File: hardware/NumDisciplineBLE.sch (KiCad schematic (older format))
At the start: 22 parts, among them J2 SWD, J3 Ex_Bat, J4 Ex_USB, Q1 AO3407, Q2 AO3407, U1 E73-2G4M08S1C, U2 XC6220B331MR-G, U3 TP4054, U5 ATmega32A-P, X1 32.768kHz

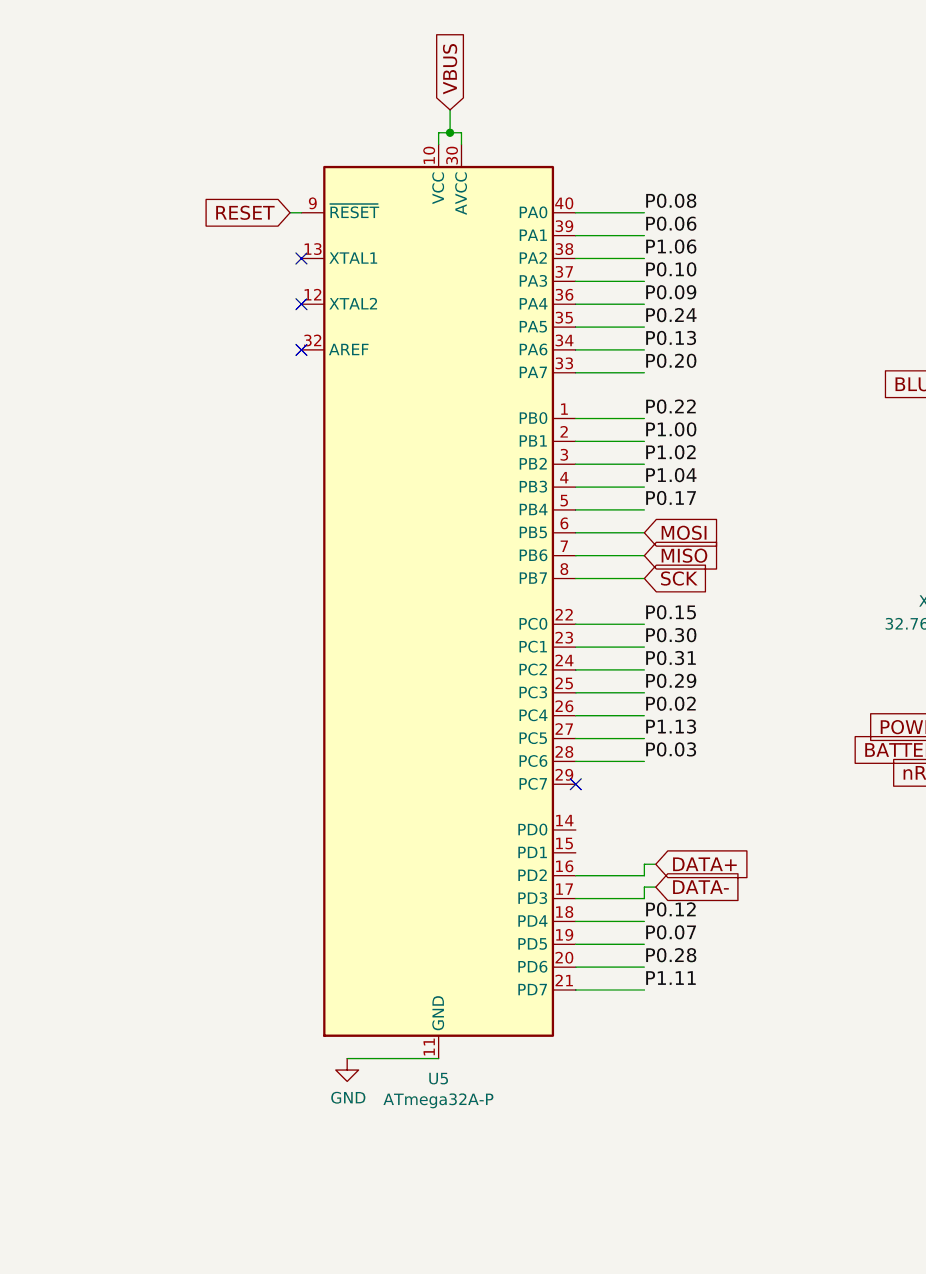
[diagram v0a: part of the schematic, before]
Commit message: basic layout done
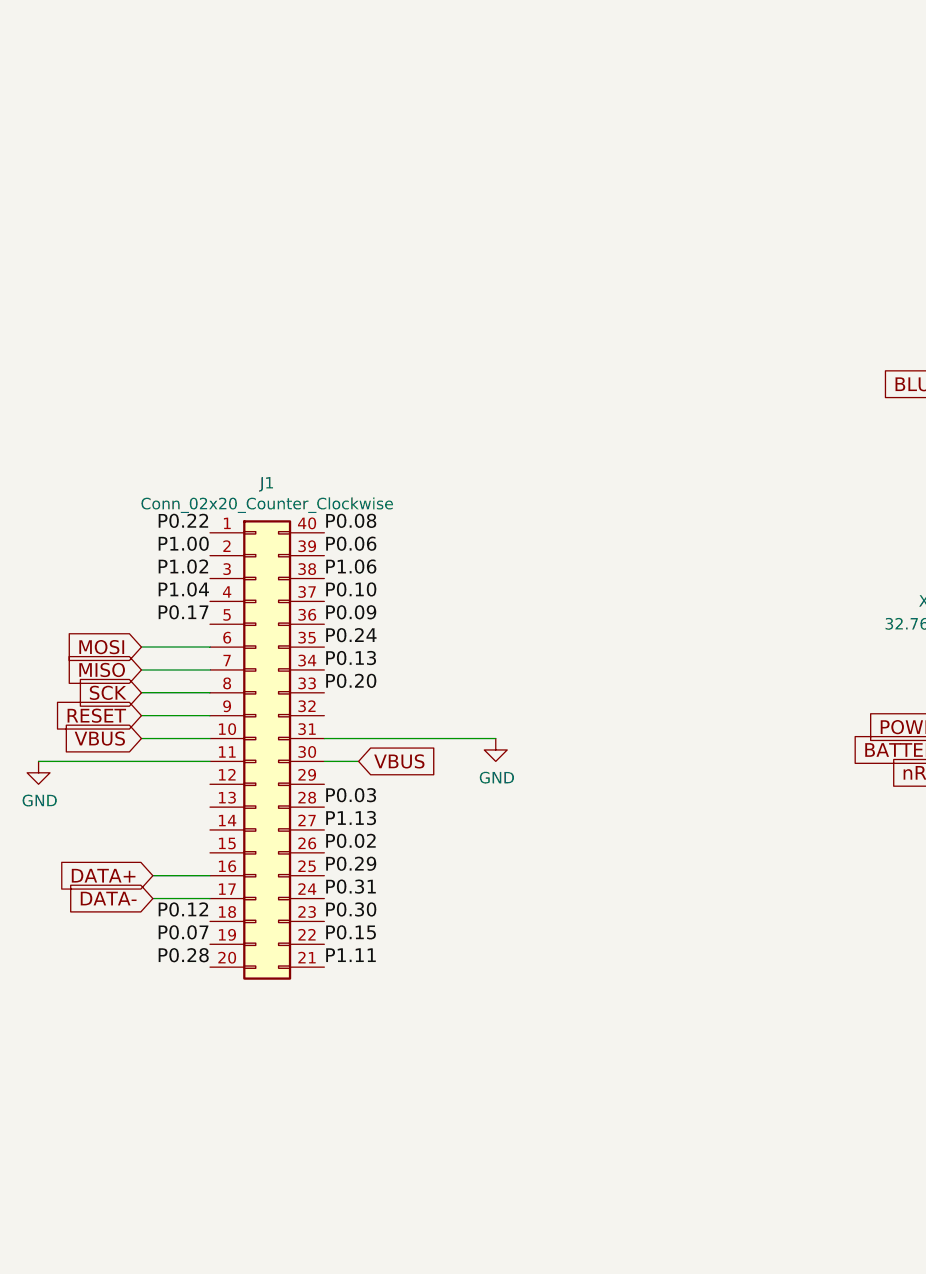
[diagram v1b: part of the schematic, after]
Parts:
- removed U5: ATmega32A-P, Package_DIP:DIP-40_W15.24mm, symbol MCU_Microchip_ATmega:ATmega32A-P
- added J1: Conn_02x20_Counter_Clockwise, nrfmicro:2x20_P2.54mm_Vertical_SMD_reversed, symbol Connector_Generic:Conn_02x20_Counter_Clockwise
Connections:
- net DATA+: now also J1.16 (Pin_16)
- net DATA-: now also J1.17 (Pin_17)
- net GND: now also J1.11 (Pin_11), J1.31 (Pin_31)
- net MISO: now also J1.7 (Pin_7)
- net MOSI: now also J1.6 (Pin_6)
- net P0.02: now also J1.26 (Pin_26)
- net P0.03: now also J1.28 (Pin_28)
- net P0.06: now also J1.39 (Pin_39)
- net P0.07: now also J1.19 (Pin_19)
- net P0.08: now also J1.40 (Pin_40)
- net P0.09: now also J1.36 (Pin_36)
- net P0.10: now also J1.37 (Pin_37)
- net P0.12: now also J1.18 (Pin_18)
- net P0.13: now also J1.34 (Pin_34)
- net P0.15: now also J1.22 (Pin_22)
- net P0.17: now also J1.5 (Pin_5)
- net P0.20: now also J1.33 (Pin_33)
- net P0.22: now also J1.1 (Pin_1)
- net P0.24: now also J1.35 (Pin_35)
- net P0.28: now also J1.20 (Pin_20)
- net P0.29: now also J1.25 (Pin_25)
- net P0.30: now also J1.23 (Pin_23)
- net P0.31: now also J1.24 (Pin_24)
- net P1.00: now also J1.2 (Pin_2)
- net P1.02: now also J1.3 (Pin_3)
- net P1.04: now also J1.4 (Pin_4)
- net P1.06: now also J1.38 (Pin_38)
- net P1.11: now also J1.21 (Pin_21)
- net P1.13: now also J1.27 (Pin_27)
- net RESET: now also J1.9 (Pin_9)
- net SCK: now also J1.8 (Pin_8)
- net VBUS: now also J1.10 (Pin_10), J1.30 (Pin_30)
- no-connect marks 4 -> 0
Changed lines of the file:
@@
 Wire Wire Line
 	3000 3050 3525 3050
+Wire Wire Line
+	-2150 2600 -2450 2600
+Wire Wire Line
+	-2450 2500 -2150 2500
+Wire Wire Line
+	-2150 2400 -2450 2400
+Wire Wire Line
+	-2450 2300 -2150 2300
+Text Label -2150 3500 2    60   ~ 0
+P0.12
+Text Label -2150 3600 2    60   ~ 0
+P0.07
+Text Label -2150 3700 2    60   ~ 0
+P0.28
+Text GLabel -2400 3400 0    60   Input ~ 0
+DATA-
+Text GLabel -2400 3300 0    60   Input ~ 0
+DATA+
 $Comp
-L MCU_Microchip_ATmega:ATmega32A-P U5
-U 1 1 5FA7B77E
-P -1150 2100
-F 0 "U5" H -1150 11  50  0000 C CNN
-F 1 "ATmega32A-P" H -1150 -80 50  0000 C CNN
-F 2 "Package_DIP:DIP-40_W15.24mm" H -1150 2100 50  0001 C CIN
-F 3 "http://ww1.microchip.com/downloads/en/DeviceDoc/atmel-8155-8-bit-microcontroller-avr-atmega32a_datasheet.pdf" H -1150 2100 50  0001 C CNN
-	1    -1150 2100
+L power:GND #PWR0111
+U 1 1 5FA32D25
+P -2900 2800
+F 0 "#PWR0111" H -2900 2550 50  0001 C CNN
+F 1 "GND" H -2895 2627 50  0000 C CNN
+F 2 "" H -2900 2800 50  0001 C CNN
+F 3 "" H -2900 2800 50  0001 C CNN
+	1    -2900 2800
 	1    0    0    -1
 $EndComp
-Text GLabel -200 3250 2    60   Input ~ 0
-DATA+
-Text GLabel -200 3350 2    60   Input ~ 0
-DATA-
+Text GLabel -2450 2700 0    60   Input ~ 0
+VBUS
+Text GLabel -2450 2600 0    60   Input ~ 0
+RESET
+Text Label -2150 2100 2    60   ~ 0
+P1.04
+Text Label -2150 2000 2    60   ~ 0
+P1.02
+Text Label -2150 1900 2    60   ~ 0
+P1.00
+Text Label -2150 1800 2    60   ~ 0
+P0.22
+Text GLabel -2450 2500 0    60   Input ~ 0
+SCK
+Text GLabel -2450 2400 0    60   Input ~ 0
+MISO
+Text GLabel -2450 2300 0    60   Input ~ 0
+MOSI
+Text Label -2150 2200 2    60   ~ 0
+P0.17
 Wire Wire Line
-	-250 3300 -550 3300
+	-2450 2700 -2150 2700
 Wire Wire Line
-	-250 3400 -550 3400
+	-2150 2800 -2900 2800
+Wire Wire Line
+	-2150 3300 -2400 3300
+Wire Wire Line
+	-2150 3400 -2400 3400
 $Comp
-L power:GND #PWR0118
-U 1 1 5FA87E35
-P -1550 4100
-F 0 "#PWR0118" H -1550 3850 50  0001 C CNN
-F 1 "GND" H -1545 3927 50  0000 C CNN
-F 2 "" H -1550 4100 50  0001 C CNN
-F 3 "" H -1550 4100 50  0001 C CNN
-	1    -1550 4100
+L Connector_Generic:Conn_02x20_Counter_Clockwise J1
+U 1 1 5FAA6BCE
+P -1950 2700
+F 0 "J1" H -1900 3817 50  0000 C CNN
+F 1 "Conn_02x20_Counter_Clockwise" H -1900 3726 50  0000 C CNN
+F 2 "nrfmicro:2x20_P2.54mm_Vertical_SMD_reversed" H -1950 2700 50  0001 C CNN
+F 3 "~" H -1950 2700 50  0001 C CNN
+	1    -1950 2700
+	1    0    0    -1
+$EndComp
+Text GLabel -1500 2800 2    60   Input ~ 0
+VBUS
+Text Label -1650 3700 0    60   ~ 0
+P1.11
+Text Label -1650 3600 0    60   ~ 0
+P0.15
+Text Label -1650 3500 0    60   ~ 0
+P0.30
+Text Label -1650 3400 0    60   ~ 0
+P0.31
+Text Label -1650 3300 0    60   ~ 0
+P0.29
+Text Label -1650 3200 0    60   ~ 0
+P0.02
+Text Label -1650 3000 0    60   ~ 0
+P0.03
+Text Label -1650 3100 0    60   ~ 0
+P1.13
+Text Label -1650 2500 0    60   ~ 0
+P0.20
+Text Label -1650 2200 0    60   ~ 0
+P0.09
+Text Label -1650 2100 0    60   ~ 0
+P0.10
+Text Label -1650 2400 0    60   ~ 0
+P0.13
+Text Label -1650 2000 0    60   ~ 0
+P1.06
+Text Label -1650 2300 0    60   ~ 0
+P0.24
+Text Label -1650 1800 0    60   ~ 0
+P0.08
+Text Label -1650 1900 0    60   ~ 0
+P0.06
+Wire Wire Line
+	-1500 2800 -1650 2800
+$Comp
+L power:GND #PWR0113
+U 1 1 5FAACC3A
+P -900 2700
+F 0 "#PWR0113" H -900 2450 50  0001 C CNN
+F 1 "GND" H -895 2527 50  0000 C CNN
+F 2 "" H -900 2700 50  0001 C CNN
+F 3 "" H -900 2700 50  0001 C CNN
+	1    -900 2700
 	1    0    0    -1
 $EndComp
 Wire Wire Line
-	-1550 4100 -1150 4100
-Text GLabel -1800 400  0    60   Input ~ 0
-RESET
-Wire Wire Line
-	-1750 400  -1800 400
-Wire Wire Line
-	-1050 100  -1050 50
-Wire Wire Line
-	-1050 50   -1100 50
-Wire Wire Line
-	-1150 50   -1150 100
-Text Label -250 2200 0    60   ~ 0
-P0.15
-Text Label -250 1700 0    60   ~ 0
-P0.17
-Text Label -250 1100 0    60   ~ 0
-P0.20
-Text Label -250 800  0    60   ~ 0
-P0.09
-Text Label -250 700  0    60   ~ 0
-P0.10
-Text Label -250 1000 0    60   ~ 0
-P0.13
-Text Label -250 600  0    60   ~ 0
-P1.06
-Text Label -250 900  0    60   ~ 0
-P0.24
-Wire Wire Line
-	-250 400  -550 400
-Wire Wire Line
-	-250 500  -550 500
-Wire Wire Line
-	-250 600  -550 600
-Wire Wire Line
-	-250 700  -550 700
-Wire Wire Line
-	-250 800  -550 800
-Wire Wire Line
-	-250 900  -550 900
-Wire Wire Line
-	-250 1000 -550 1000
-Wire Wire Line
-	-250 1100 -550 1100
-Text Label -250 3800 0    60   ~ 0
-P1.11
-Text Label -250 2300 0    60   ~ 0
-P0.30
-Text Label -250 2400 0    60   ~ 0
-P0.31
-Text Label -250 2500 0    60   ~ 0
-P0.29
-Text Label -250 2600 0    60   ~ 0
-P0.02
-Text Label -250 2800 0    60   ~ 0
-P0.03
-Text Label -250 3700 0    60   ~ 0
-P0.28
-Text Label -250 2700 0    60   ~ 0
-P1.13
-Wire Wire Line
-	-250 1300 -550 1300
-Wire Wire Line
-	-250 1400 -550 1400
-Wire Wire Line
-	-250 1500 -550 1500
-Wire Wire Line
-	-250 1600 -550 1600
-Wire Wire Line
-	-250 1700 -550 1700
-Wire Wire Line
-	-250 2200 -550 2200
-Wire Wire Line
-	-250 2300 -550 2300
-Wire Wire Line
-	-250 2400 -550 2400
-Text Label -250 400  0    60   ~ 0
-P0.08
-Text Label -250 500  0    60   ~ 0
-P0.06
-Text GLabel -250 1800 2    60   Input ~ 0
-MOSI
-Text GLabel -250 1900 2    60   Input ~ 0
-MISO
-Text GLabel -250 2000 2    60   Input ~ 0
-SCK
-Wire Wire Line
-	-250 1800 -550 1800
-Wire Wire Line
-	-250 1900 -550 1900
-Wire Wire Line
-	-250 2000 -550 2000
-Text Label -250 1300 0    60   ~ 0
-P0.22
-Text Label -250 1400 0    60   ~ 0
-P1.00
-Text Label -250 1500 0    60   ~ 0
-P1.02
-Text Label -250 1600 0    60   ~ 0
-P1.04
-Text Label -250 3600 0    60   ~ 0
-P0.07
-Text Label -250 3500 0    60   ~ 0
-P0.12
-Wire Wire Line
-	-250 3400 -250 3350
-Wire Wire Line
-	-250 3350 -200 3350
-Wire Wire Line
-	-250 3300 -250 3250
-Wire Wire Line
-	-250 3250 -200 3250
-Wire Wire Line
-	-250 3500 -550 3500
-Wire Wire Line
-	-250 3600 -550 3600
-Wire Wire Line
-	-250 3700 -550 3700
-Wire Wire Line
-	-250 3800 -550 3800
-Wire Wire Line
-	-250 2800 -550 2800
-Wire Wire Line
-	-250 2700 -550 2700
-Wire Wire Line
-	-250 2600 -550 2600
-Wire Wire Line
-	-250 2500 -550 2500
-NoConn ~ -1750 600
-NoConn ~ -1750 800
-NoConn ~ -1750 1000
-NoConn ~ -550 2900
-Text GLabel -1100 -50  1    60   Input ~ 0
-VBUS
-Wire Wire Line
-	-1100 -50  -1100 50
-Connection ~ -1100 50
-Wire Wire Line
-	-1100 50   -1150 50
+	-1650 2700 -900 2700
 $EndSCHEMATC
